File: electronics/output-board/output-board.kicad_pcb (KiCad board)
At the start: 4 copper layers, 105.2 x 77.5 mm, 95 parts, among them J1 Conn_01x02_Male, J10 Conn_01x02_Male, J11 Conn_01x02_Male, J12 Conn_01x02_Male, J13 Conn_01x02_Male, J14 Arming switch, J15 Conn_01x02_Male, J16 Conn_01x02_Male, J17 Conn_01x02_Male, J18 Conn_01x02_Male, J19 Extra IO, J2 Conn_01x02_Male, J3 12V In, J4 Conn_01x02, J5 SWD Header, J6 Conn_01x02, J7 Conn_01x02_Male, J8 Conn_01x02_Male, J9 Conn_01x02_Male, SW1 SW_Push_Dual, U1 MAX33012EASA+, U2 LD3985M33R_SOT23, U3 STM32F105VBH6, Y1 25MHz 9pF

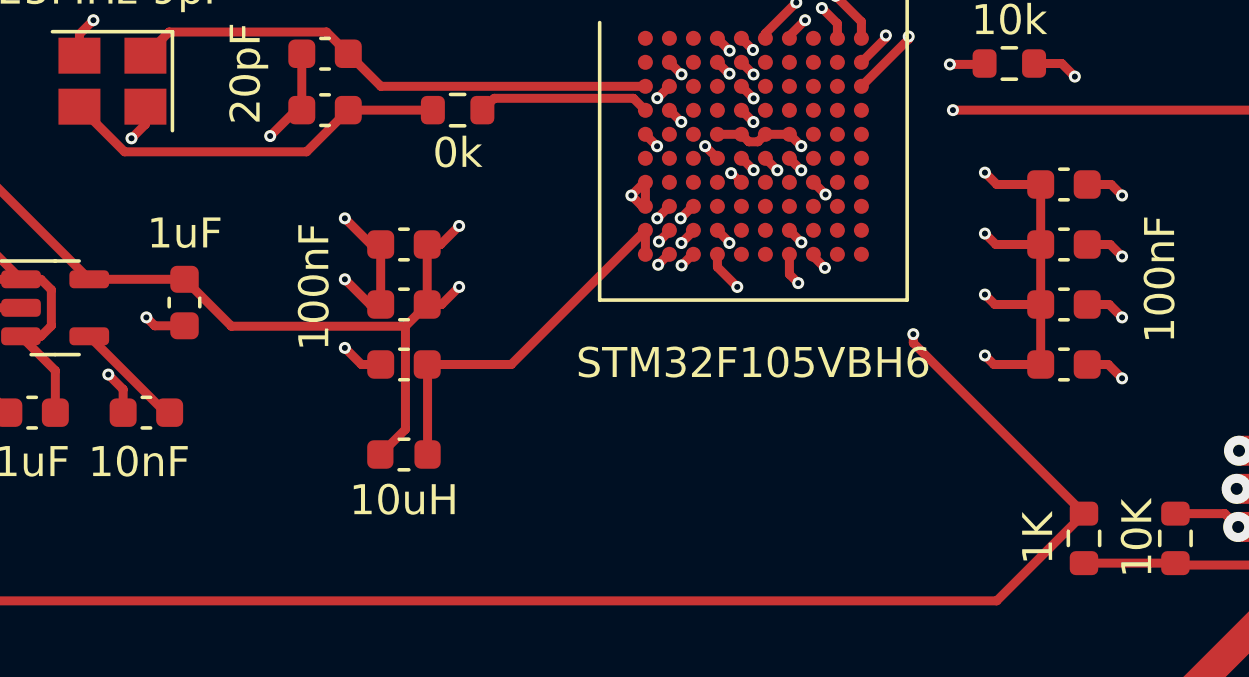
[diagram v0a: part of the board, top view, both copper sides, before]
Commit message: minor changes to output board
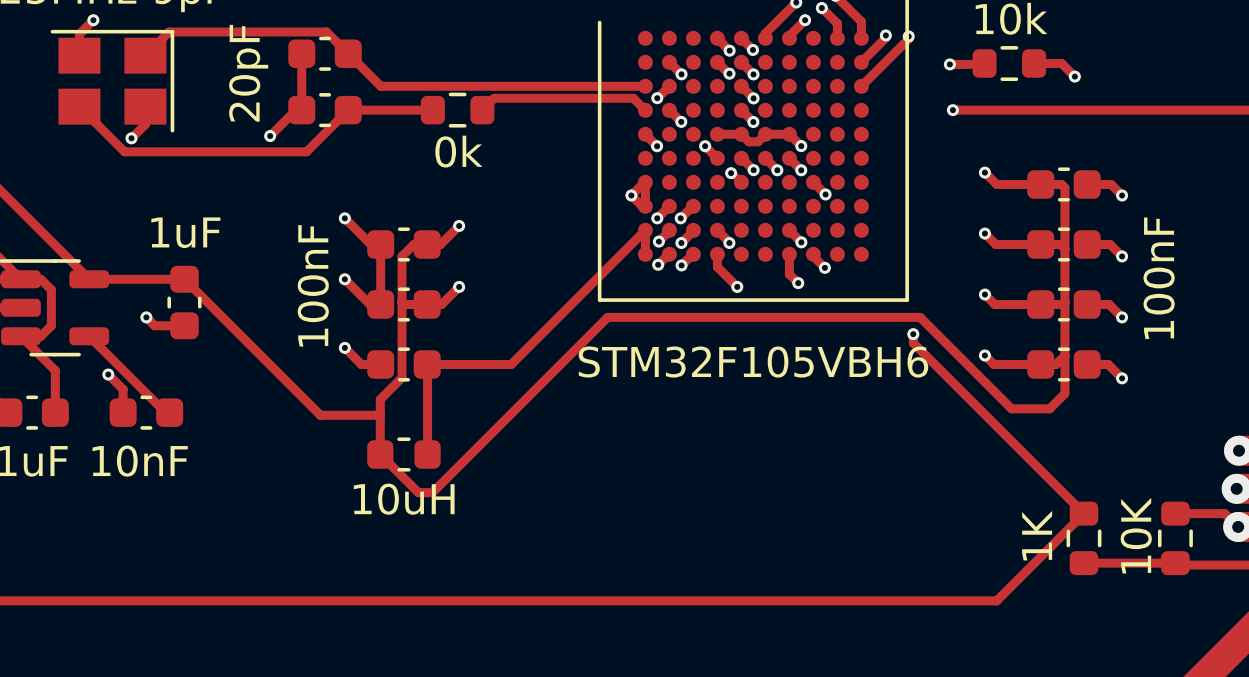
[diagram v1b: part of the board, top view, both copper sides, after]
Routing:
- net +3V3: track 131.8 -> 146.2 mm
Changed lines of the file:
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@@
   (segment (start 71.249 74.549) (end 71.109 74.549) (width 0.3) (layer "F.Cu") (net 51))
   (segment (start 71.114 74.549) (end 71.249 74.549) (width 0.3) (layer "F.Cu") (net 51))
+  (segment (start 100.98 66.944) (end 101.092 67.056) (width 0.3) (layer "F.Cu") (net 52))
   (segment (start 91.1078 66.07165) (end 91.505748 66.469598) (width 0.3) (layer "F.Cu") (net 52))
+  (segment (start 101.092 72.644) (end 100.792 72.944) (width 0.3) (layer "F.Cu") (net 52))
   (segment (start 71.744 70.104) (end 68.569 70.104) (width 0.3) (layer "F.Cu") (net 52))
+  (segment (start 101.092 73.914) (end 100.584 74.422) (width 0.3) (layer "F.Cu") (net 52))
+  (segment (start 100.948 68.944) (end 101.092 69.088) (width 0.3) (layer "F.Cu") (net 52))
   (segment (start 89.5078 66.0712) (end 89.503324 66.0712) (width 0.3) (layer "F.Cu") (net 52))
   (segment (start 80.313 70.944) (end 80.899 70.358) (width 0.3) (layer "F.Cu") (net 52))
   (segment (start 68.569 70.104) (end 59.806499 61.341499) (width 0.3) (layer "F.Cu") (net 52))
-  (segment (start 100.284 66.944) (end 100.284 68.944) (width 0.3) (layer "F.Cu") (net 52))
+  (segment (start 78.2715 74.6365) (end 78.2715 75.944) (width 0.3) (layer "F.Cu") (net 52))
   (segment (start 60.568647 56.144353) (end 61.14661 56.144353) (width 0.3) (layer "F.Cu") (net 52))
+  (segment (start 101.092 67.056) (end 101.092 69.088) (width 0.3) (layer "F.Cu") (net 52))
   (segment (start 79.834 68.944) (end 80.281 68.944) (width 0.3) (layer "F.Cu") (net 52))
+  (segment (start 78.2715 74.108806) (end 78.2715 74.6365) (width 0.3) (layer "F.Cu") (net 52))
+  (segment (start 76.2765 74.6365) (end 78.2715 74.6365) (width 0.3) (layer "F.Cu") (net 52))
+  (segment (start 71.744 70.104) (end 76.2765 74.6365) (width 0.3) (layer "F.Cu") (net 52))
+  (segment (start 79.392 68.944) (end 78.994 69.342) (width 0.3) (layer "F.Cu") (net 52))
+  (segment (start 78.994 73.386306) (end 78.2715 74.108806) (width 0.3) (layer "F.Cu") (net 52))
   (segment (start 98.821 66.944) (end 98.425 66.548) (width 0.3) (layer "F.Cu") (net 52))
   (segment (start 100.284 68.944) (end 98.789 68.944) (width 0.3) (layer "F.Cu") (net 52))
   (segment (start 100.284 66.944) (end 98.821 66.944) (width 0.3) (layer "F.Cu") (net 52))
   (segment (start 87.917627 64.4712) (end 88.303886 64.857459) (width 0.3) (layer "F.Cu") (net 52))
-  (segment (start 100.284 68.944) (end 100.284 70.944) (width 0.3) (layer "F.Cu") (net 52))
+  (segment (start 79.072 70.944) (end 78.994 70.866) (width 0.3) (layer "F.Cu") (net 52))
+  (segment (start 100.284 68.944) (end 100.948 68.944) (width 0.3) (layer "F.Cu") (net 52))
   (segment (start 91.9078 66.0712) (end 91.9078 66.075129) (width 0.3) (layer "F.Cu") (net 52))
   (segment (start 98.789 68.944) (end 98.425 68.58) (width 0.3) (layer "F.Cu") (net 52))
   (segment (start 98.725 72.944) (end 98.425 72.644) (width 0.3) (layer "F.Cu") (net 52))
   (segment (start 87.9078 62.8712) (end 87.910484 62.8712) (width 0.3) (layer "F.Cu") (net 52))
+  (segment (start 100.284 66.944) (end 100.98 66.944) (width 0.3) (layer "F.Cu") (net 52))
+  (segment (start 100.284 70.944) (end 101.014 70.944) (width 0.3) (layer "F.Cu") (net 52))
   (segment (start 100.284 72.944) (end 98.725 72.944) (width 0.3) (layer "F.Cu") (net 52))
+  (segment (start 100.792 72.944) (end 100.284 72.944) (width 0.3) (layer "F.Cu") (net 52))
+  (segment (start 100.584 74.422) (end 99.314 74.422) (width 0.3) (layer "F.Cu") (net 52))
   (segment (start 59.806499 56.906501) (end 60.568647 56.144353) (width 0.3) (layer "F.Cu") (net 52))
+  (segment (start 101.014 70.944) (end 101.092 70.866) (width 0.3) (layer "F.Cu") (net 52))
   (segment (start 59.806499 61.341499) (end 59.806499 56.906501) (width 0.3) (layer "F.Cu") (net 52))
   (segment (start 90.3078 66.0712) (end 90.321191 66.0712) (width 0.3) (layer "F.Cu") (net 52))
   (segment (start 91.9078 66.075129) (end 92.303036 66.470365) (width 0.3) (layer "F.Cu") (net 52))
   (segment (start 100.284 70.944) (end 98.757 70.944) (width 0.3) (layer "F.Cu") (net 52))
-  (segment (start 73.30852 71.66852) (end 79.10948 71.66852) (width 0.3) (layer "F.Cu") (net 52))
   (segment (start 98.757 70.944) (end 98.425 70.612) (width 0.3) (layer "F.Cu") (net 52))
-  (segment (start 79.10948 71.66852) (end 79.834 70.944) (width 0.3) (layer "F.Cu") (net 52))
-  (segment (start 71.744 70.104) (end 73.30852 71.66852) (width 0.3) (layer "F.Cu") (net 52))
+  (segment (start 85.852 71.374) (end 80.01 77.216) (width 0.3) (layer "F.Cu") (net 52))
+  (segment (start 101.092 72.644) (end 101.092 73.914) (width 0.3) (layer "F.Cu") (net 52))
+  (segment (start 78.994 69.342) (end 78.994 70.866) (width 0.3) (layer "F.Cu") (net 52))
+  (segment (start 80.01 77.216) (end 79.5435 77.216) (width 0.3) (layer "F.Cu") (net 52))
+  (segment (start 101.092 69.088) (end 101.092 70.866) (width 0.3) (layer "F.Cu") (net 52))
   (segment (start 80.281 68.944) (end 80.899 68.326) (width 0.3) (layer "F.Cu") (net 52))
-  (segment (start 78.2715 75.944) (end 79.10948 75.10602) (width 0.3) (layer "F.Cu") (net 52))
+  (segment (start 96.266 71.374) (end 85.852 71.374) (width 0.3) (layer "F.Cu") (net 52))
+  (segment (start 79.834 68.944) (end 79.392 68.944) (width 0.3) (layer "F.Cu") (net 52))
   (segment (start 90.321191 66.0712) (end 90.715667 66.465676) (width 0.3) (layer "F.Cu") (net 52))
-  (segment (start 100.284 70.944) (end 100.284 72.944) (width 0.3) (layer "F.Cu") (net 52))
-  (segment (start 79.834 68.944) (end 79.834 70.944) (width 0.3) (layer "F.Cu") (net 52))
   (segment (start 79.834 70.944) (end 80.313 70.944) (width 0.3) (layer "F.Cu") (net 52))
+  (segment (start 78.994 70.866) (end 78.994 73.386306) (width 0.3) (layer "F.Cu") (net 52))
   (segment (start 91.1078 66.0712) (end 91.1078 66.07165) (width 0.3) (layer "F.Cu") (net 52))
+  (segment (start 99.314 74.422) (end 96.266 71.374) (width 0.3) (layer "F.Cu") (net 52))
   (segment (start 87.9078 64.4712) (end 87.917627 64.4712) (width 0.3) (layer "F.Cu") (net 52))
-  (segment (start 79.10948 75.10602) (end 79.10948 71.66852) (width 0.3) (layer "F.Cu") (net 52))
   (segment (start 89.503324 66.0712) (end 89.098511 65.666387) (width 0.3) (layer "F.Cu") (net 52))
+  (segment (start 79.5435 77.216) (end 78.2715 75.944) (width 0.3) (layer "F.Cu") (net 52))
+  (segment (start 101.092 70.866) (end 101.092 72.644) (width 0.3) (layer "F.Cu") (net 52))
   (segment (start 87.910484 62.8712) (end 88.311746 63.272462) (width 0.3) (layer "F.Cu") (net 52))
+  (segment (start 79.834 70.944) (end 79.072 70.944) (width 0.3) (layer "F.Cu") (net 52))
   (via (at 90.715667 66.465676) (size 0.4) (drill 0.2) (layers "F.Cu" "B.Cu") (net 52))
   (via (at 91.505748 66.469598) (size 0.4) (drill 0.2) (layers "F.Cu" "B.Cu") (net 52))
@@
   (segment (start 92.380671 66.548) (end 92.303036 66.470365) (width 0.3) (layer "In2.Cu") (net 52))
   (segment (start 97.917 67.818) (end 98.425 68.326) (width 0.3) (layer "In2.Cu") (net 52))
-  (segment (start 81.026 70.231) (end 89.661294 70.231) (width 0.3) (layer "In2.Cu") (net 52))
   (segment (start 91.505748 66.469598) (end 91.505748 66.486748) (width 0.3) (layer "In2.Cu") (net 52))
   (segment (start 95.885 68.326) (end 92.075 68.326) (width 0.3) (layer "In2.Cu") (net 52))
@@
   (segment (start 98.425 70.612) (end 98.171 70.612) (width 0.3) (layer "In2.Cu") (net 52))
   (segment (start 98.425 68.326) (end 98.425 68.58) (width 0.3) (layer "In2.Cu") (net 52))
-  (segment (start 92.513783 69.781489) (end 95.376294 72.644) (width 0.3) (layer "In2.Cu") (net 52))
   (segment (start 89.098511 65.666387) (end 89.098511 66.335267) (width 0.3) (layer "In2.Cu") (net 52))
   (segment (start 92.904805 69.273489) (end 95.054489 69.273489) (width 0.3) (layer "In2.Cu") (net 52))
-  (segment (start 90.110805 69.781489) (end 92.513783 69.781489) (width 0.3) (layer "In2.Cu") (net 52))
   (segment (start 98.171 70.612) (end 95.885 68.326) (width 0.3) (layer "In2.Cu") (net 52))
   (segment (start 88.311746 63.272462) (end 85.952538 63.272462) (width 0.3) (layer "In2.Cu") (net 52))
@@
   (segment (start 98.425 66.548) (end 92.380671 66.548) (width 0.3) (layer "In2.Cu") (net 52))
   (segment (start 92.837 67.818) (end 97.917 67.818) (width 0.3) (layer "In2.Cu") (net 52))
-  (segment (start 89.661294 70.231) (end 90.110805 69.781489) (width 0.3) (layer "In2.Cu") (net 52))
   (segment (start 95.054489 69.273489) (end 98.425 72.644) (width 0.3) (layer "In2.Cu") (net 52))
-  (segment (start 95.376294 72.644) (end 98.425 72.644) (width 0.3) (layer "In2.Cu") (net 52))
   (segment (start 82.06768 64.07072) (end 81.6732 64.4652) (width 0.3) (layer "F.Cu") (net 56))
   (segment (start 87.1078 64.4712) (end 86.70732 64.07072) (width 0.3) (layer "F.Cu") (net 56))
